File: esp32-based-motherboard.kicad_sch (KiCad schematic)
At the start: 69 parts, among them J1 USB_A, J2 USB_C_Receptacle_USB2.0_16P, J3 USB_C_Receptacle_USB2.0_16P, J4 USB_C_Receptacle_USB2.0_16P, J5 Conn_01x03_Pin, J6 Conn_01x03_Pin, SW1 SW_Push, SW2 SW_Push, SW3 SW_Push, SW4 SW_Push, SW5 SW_SPST, U1 ESP32-P4_MODULE, U2 CP2102N-Axx-xQFN24, U3 ADM3053

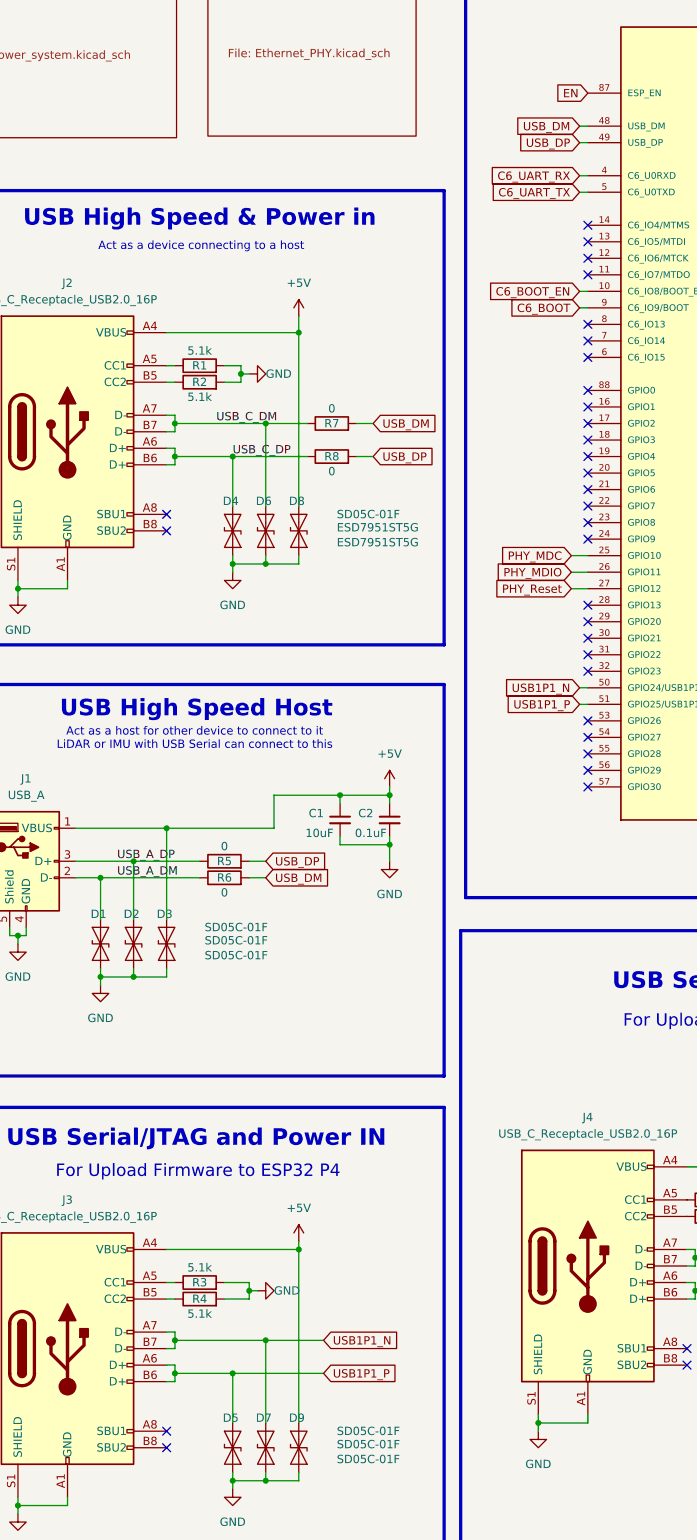
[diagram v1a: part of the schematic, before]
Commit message: Updated
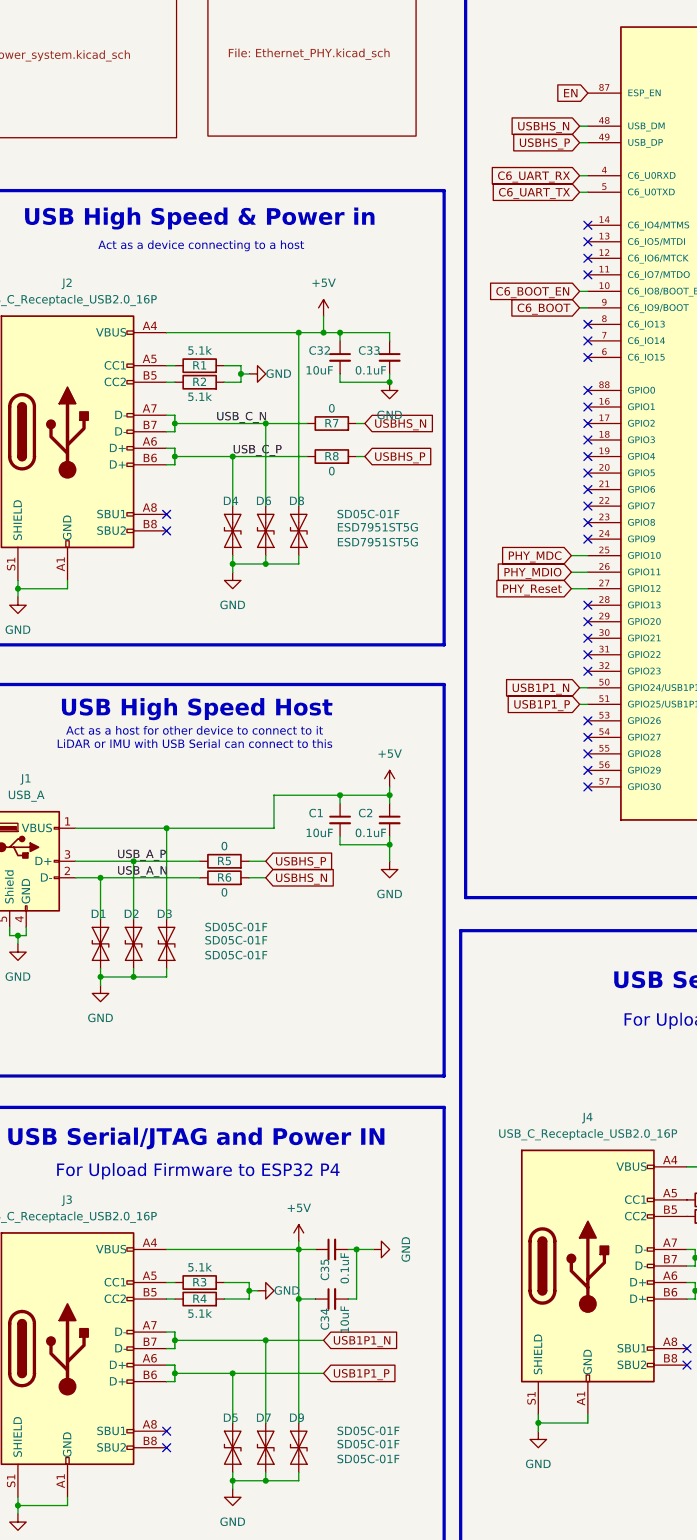
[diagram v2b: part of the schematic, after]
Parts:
- added C32, C34: 10uF, Capacitor_SMD:C_0603_1608Metric, symbol Device:C_Small
- added C33, C35: 0.1uF, Capacitor_SMD:C_0603_1608Metric, symbol Device:C_Small
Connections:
- net +5V: now also C32.1, C33.1, C34.1, C35.1
- net GND: now also C32.2, C33.2, C34.2, C35.2
- net USB_A_DM renamed USB_A_N
- net USB_A_DP renamed USB_A_P
- net USB_C_DM renamed USB_C_N
- net USB_C_DP renamed USB_C_P
- net USB_DM renamed USBHS_N
- net USB_DP renamed USBHS_P
